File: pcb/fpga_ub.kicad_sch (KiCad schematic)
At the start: 9 parts, among them J1201 Conn_02x07_Top_Bottom, U666 XC7A75T-FTG256

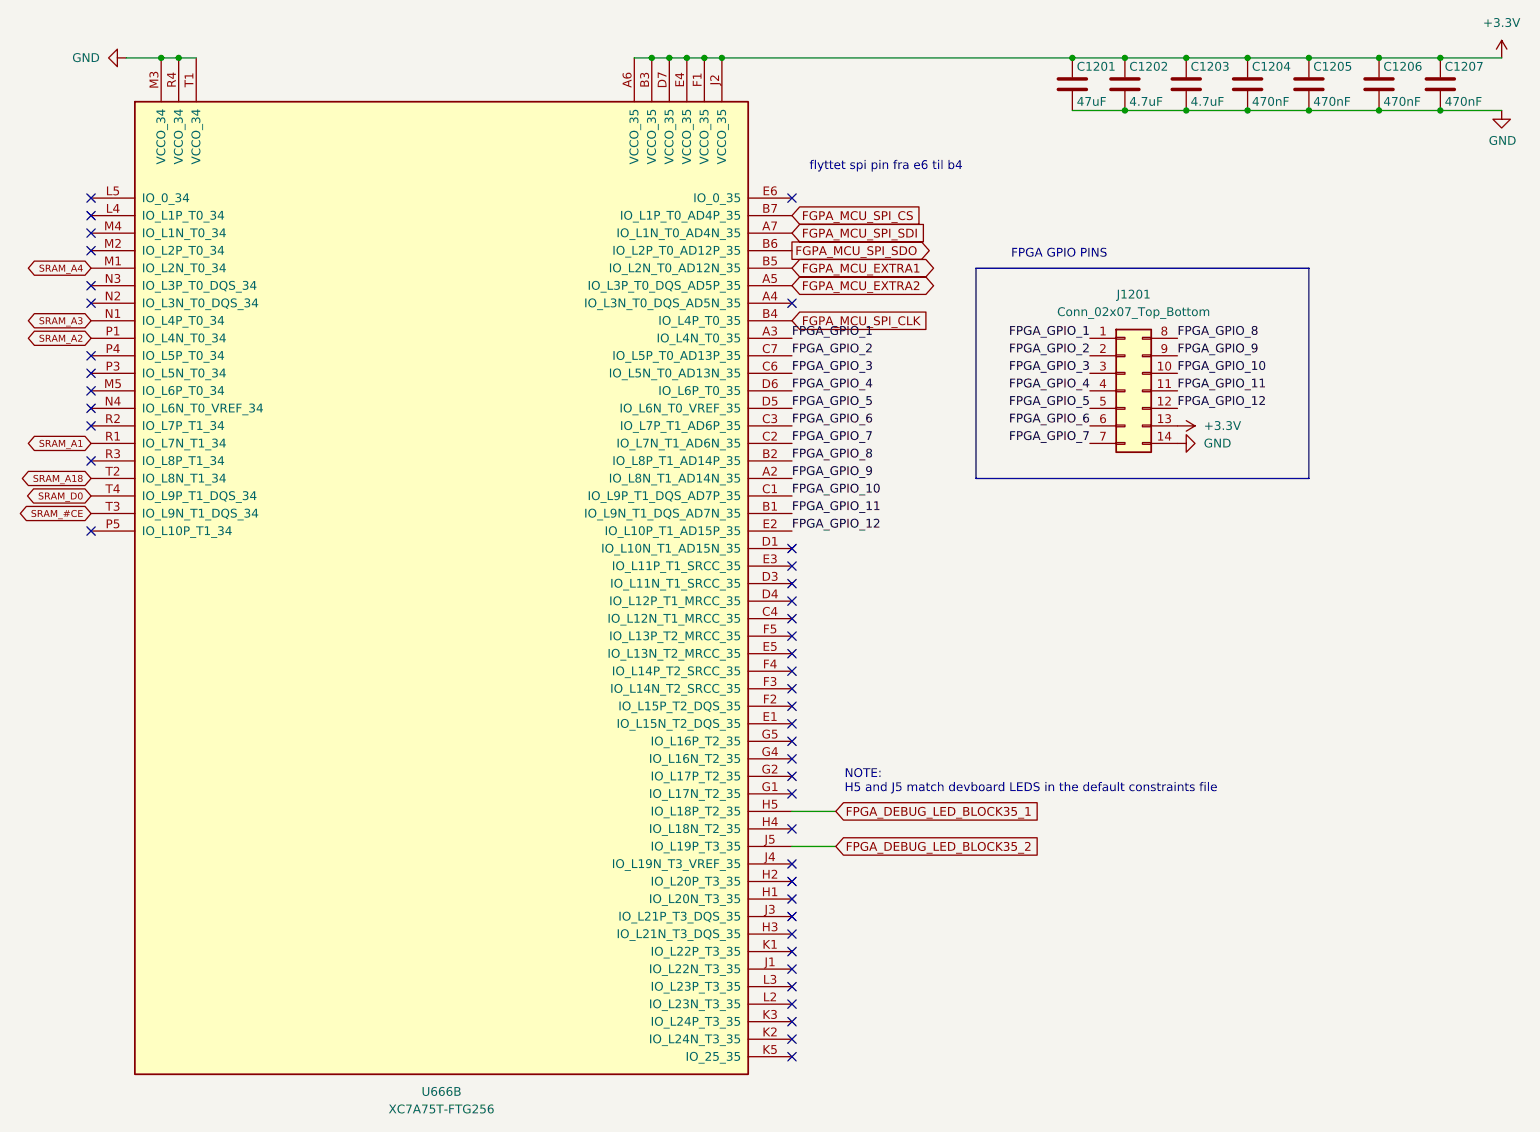
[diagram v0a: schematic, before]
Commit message: vga is live
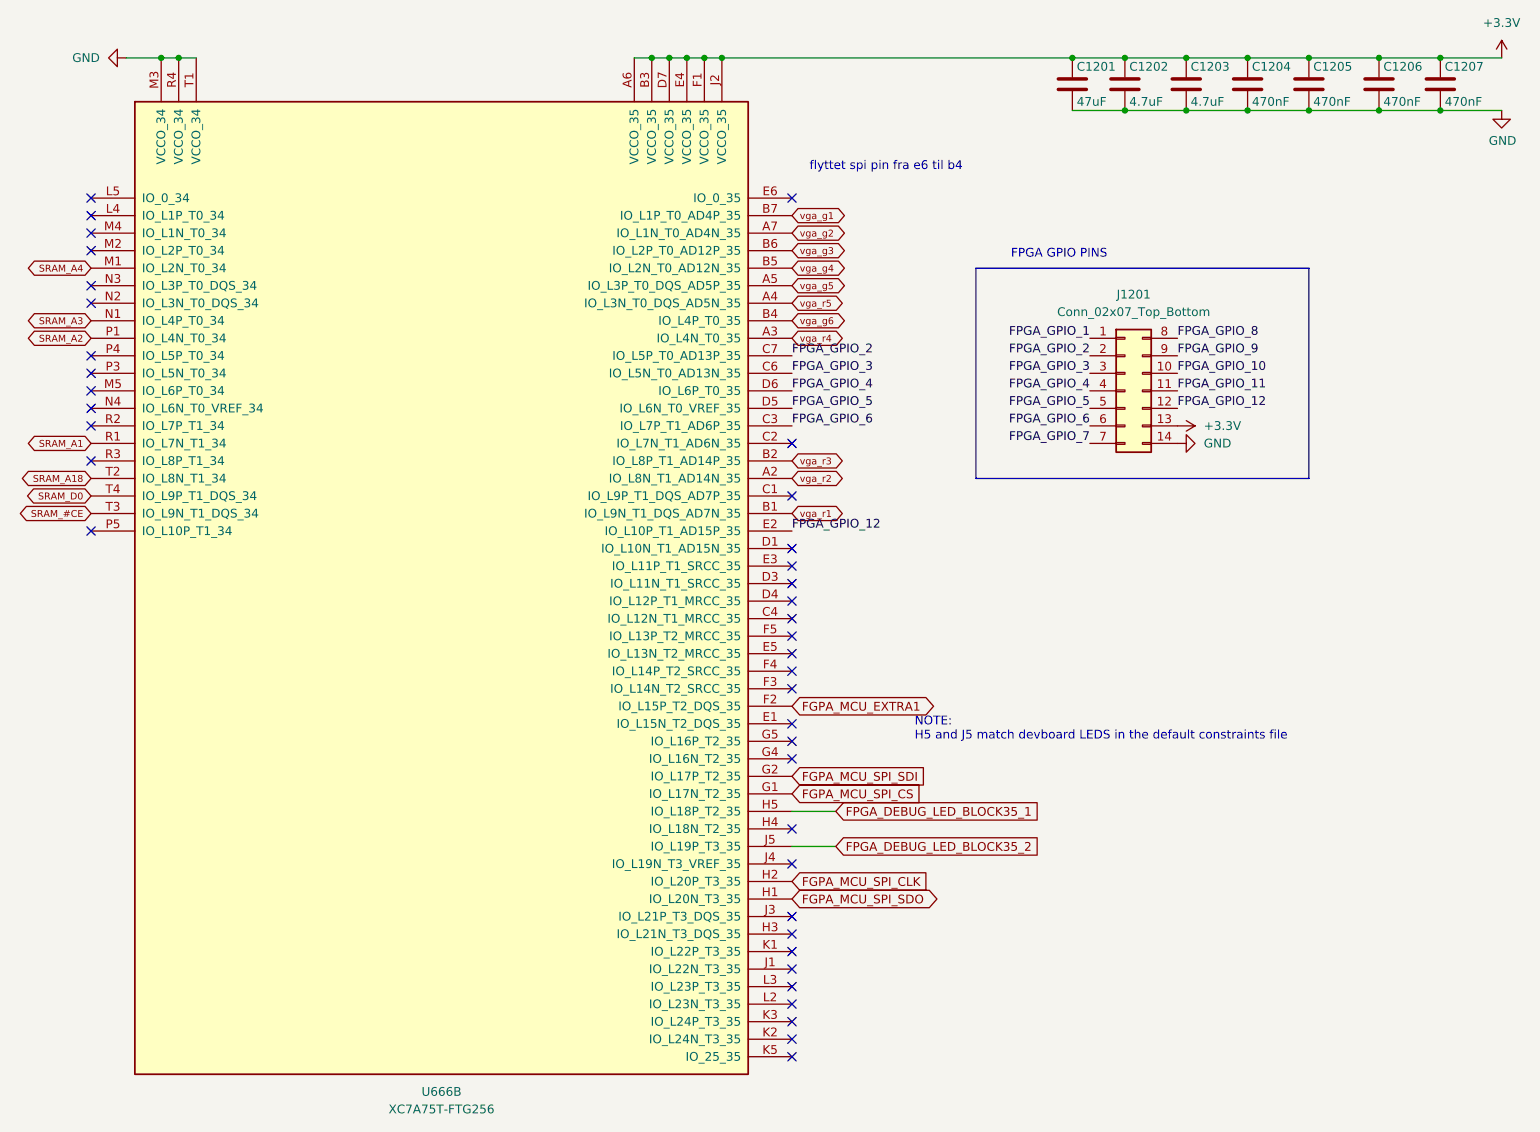
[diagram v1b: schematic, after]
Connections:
- net FGPA_MCU_EXTRA1: now also U666.F2 (IO_L15P_T2_DQS_35); no longer U666.B5 (IO_L2N_T0_AD12N_35)
- net FGPA_MCU_SPI_CLK: now also U666.H2 (IO_L20P_T3_35); no longer U666.B4 (IO_L4P_T0_35)
- net FGPA_MCU_SPI_CS: now also U666.G1 (IO_L17N_T2_35); no longer U666.B7 (IO_L1P_T0_AD4P_35)
- net FGPA_MCU_SPI_SDI: now also U666.G2 (IO_L17P_T2_35); no longer U666.A7 (IO_L1N_T0_AD4N_35)
- net FGPA_MCU_SPI_SDO: now also U666.H1 (IO_L20N_T3_35); no longer U666.B6 (IO_L2P_T0_AD12P_35)
- net FPGA_GPIO_1: no longer U666.A3 (IO_L4N_T0_35)
- net FPGA_GPIO_10: no longer U666.C1 (IO_L9P_T1_DQS_AD7P_35)
- net FPGA_GPIO_11: no longer U666.B1 (IO_L9N_T1_DQS_AD7N_35)
- net FPGA_GPIO_7: no longer U666.C2 (IO_L7N_T1_AD6N_35)
- net FPGA_GPIO_8: no longer U666.B2 (IO_L8P_T1_AD14P_35)
- net FPGA_GPIO_9: no longer U666.A2 (IO_L8N_T1_AD14N_35)
- net vga_r5: now reaches U666.A4 (IO_L3N_T0_DQS_AD5N_35)
- net FGPA_MCU_EXTRA2 renamed vga_g5
- new net vga_g1: U666.B7 (IO_L1P_T0_AD4P_35)
- new net vga_g2: U666.A7 (IO_L1N_T0_AD4N_35)
- new net vga_g3: U666.B6 (IO_L2P_T0_AD12P_35)
- new net vga_g4: U666.B5 (IO_L2N_T0_AD12N_35)
- new net vga_g6: U666.B4 (IO_L4P_T0_35)
- new net vga_r1: U666.B1 (IO_L9N_T1_DQS_AD7N_35)
- new net vga_r2: U666.A2 (IO_L8N_T1_AD14N_35)
- new net vga_r3: U666.B2 (IO_L8P_T1_AD14P_35)
- new net vga_r4: U666.A3 (IO_L4N_T0_35)
- no-connect marks 43 -> 39
